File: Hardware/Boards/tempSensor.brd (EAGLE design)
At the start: 17.4 x 17.8 mm, 6 parts, among them IC1 DS1820

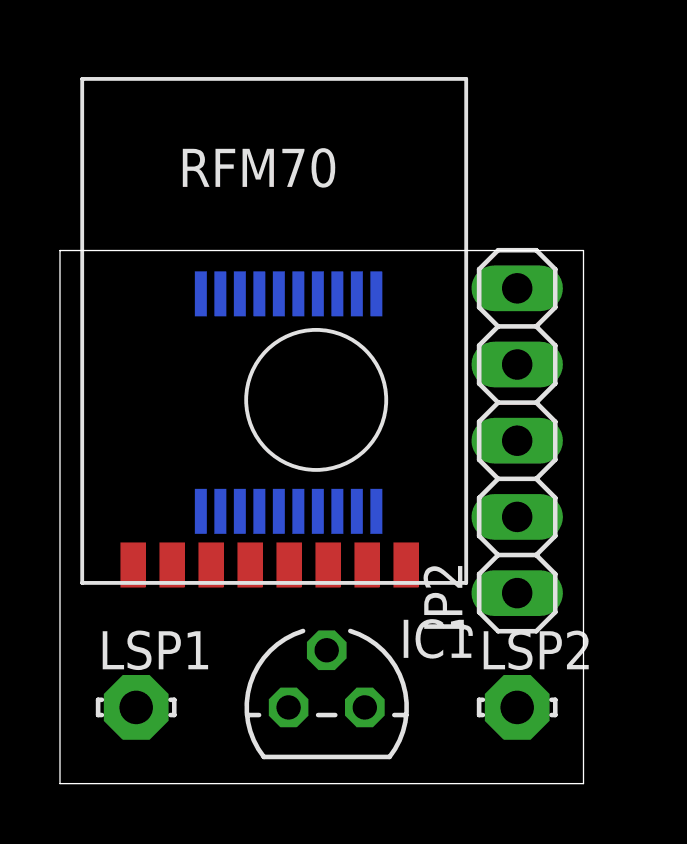
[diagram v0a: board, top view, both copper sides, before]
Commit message: a
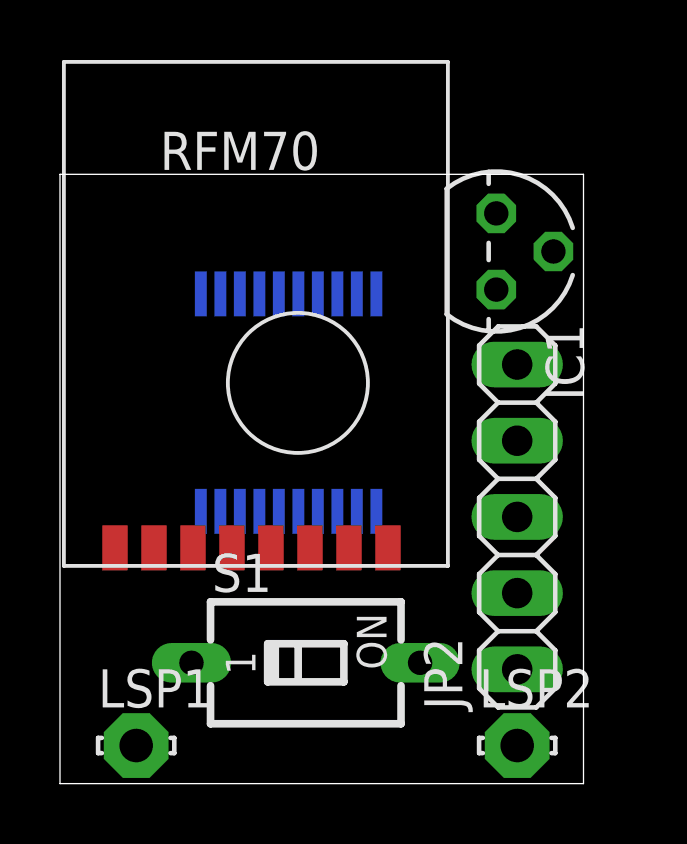
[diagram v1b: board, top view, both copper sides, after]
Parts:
- added S1: (no value), switch-dil:SD4-01
- moved IC1 16.2 mm to (14.5, 17.7), turned to 270 degrees
- moved JP2 2.54 mm to (15.2, 8.89)
- moved LSP1 1.27 mm to (2.54, 1.27)
- moved LSP2 1.27 mm to (15.2, 1.27)
- moved U$1 0.83 mm to (1.93, 22.2)
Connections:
- new net N$2: S1.2, U$2.3
- net N$5: now also S1.1
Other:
- board size 17.4 x 17.8 mm -> 17.4 x 20.3 mm
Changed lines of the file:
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@@
 <setting verticaltext="up"/>
 </settings>
-<grid distance="0.05" unitdist="inch" unit="inch" style="lines" multiple="1" display="no" altdistance="0.025" altunitdist="inch" altunit="inch"/>
+<grid distance="0.003125" unitdist="mic" unit="mm" style="lines" multiple="1" display="no" altdistance="0.025" altunitdist="inch" altunit="inch"/>
 <layers>
 <layer number="1" name="Top" color="4" fill="1" visible="yes" active="yes"/>
@@
 <plain>
 <wire x1="0" y1="0" x2="17.45" y2="0" width="0" layer="20"/>
-<wire x1="17.45" y1="0" x2="17.45" y2="17.77" width="0" layer="20"/>
-<wire x1="17.45" y1="17.77" x2="0" y2="17.77" width="0" layer="20"/>
-<wire x1="0" y1="17.77" x2="0" y2="0" width="0" layer="20"/>
+<wire x1="17.45" y1="0" x2="17.45" y2="20.31" width="0" layer="20"/>
+<wire x1="17.45" y1="20.31" x2="0" y2="20.31" width="0" layer="20"/>
+<wire x1="0" y1="20.31" x2="0" y2="0" width="0" layer="20"/>
 </plain>
 <attributes>
@@
 </autorouter>
 <elements>
-<element name="U$1" library="rfm70" package="RFM70" value="RFM70" x="2.54" y="21.59"/>
+<element name="U$1" library="rfm70" package="RFM70" value="RFM70" x="1.929840625" y="22.157171875"/>
 <element name="U$2" library="microchip" package="SSOP20" value="PIC16F690" x="7.62" y="12.7" rot="MR0"/>
-<element name="JP2" library="pinhead" package="1X05" value="Prog" x="15.24" y="11.43" rot="R90"/>
-<element name="IC1" library="ds1820" package="TO-92" value="DS1820" x="8.89" y="2.54"/>
-<element name="LSP1" library="solpad" package="LSP11" value="LSP11" x="2.54" y="2.54"/>
-<element name="LSP2" library="solpad" package="LSP11" value="LSP11" x="15.24" y="2.54"/>
+<element name="JP2" library="pinhead" package="1X05" value="Prog" x="15.24" y="8.89" rot="R90"/>
+<element name="IC1" library="ds1820" package="TO-92" value="DS1820" x="14.542675" y="17.7377375" rot="R270"/>
+<element name="LSP1" library="solpad" package="LSP11" value="LSP11" x="2.54" y="1.27"/>
+<element name="LSP2" library="solpad" package="LSP11" value="LSP11" x="15.24" y="1.27"/>
+<element name="S1" library="switch-dil" package="SD4-01" value="" x="8.192675" y="4.027234375" rot="R270">
+<attribute name="OC_NEWARK" value="unknown" x="8.192675" y="4.027234375" size="1.778" layer="27" rot="R270" display="off"/>
+<attribute name="MPN" value="" x="8.192675" y="4.027234375" size="1.778" layer="27" rot="R270" display="off"/>
+<attribute name="MF" value="" x="8.192675" y="4.027234375" size="1.778" layer="27" rot="R270" display="off"/>
+<attribute name="OC_FARNELL" value="unknown" x="8.192675" y="4.027234375" size="1.778" layer="27" rot="R270" display="off"/>
+</element>
 </elements>
 <signals>
@@
 <contactref element="IC1" pad="1"/>
 <contactref element="LSP2" pad="MP"/>
-<wire x1="10.545" y1="16.325" x2="2.44" y2="7.29" width="0" layer="19" extent="1-1"/>
-<wire x1="15.24" y1="11.43" x2="10.545" y2="16.325" width="0" layer="19" extent="1-1"/>
-<wire x1="7.62" y1="2.54" x2="15.24" y2="11.43" width="0" layer="19" extent="1-1"/>
-<wire x1="15.24" y1="2.54" x2="7.62" y2="2.54" width="0" layer="19" extent="1-1"/>
+<contactref element="S1" pad="1"/>
+<wire x1="15.24" y1="8.89" x2="10.545" y2="16.325" width="0" layer="19" extent="16-16"/>
+<wire x1="15.24" y1="1.27" x2="15.24" y2="8.89" width="0" layer="19" extent="1-1"/>
+<wire x1="14.542675" y1="19.0077375" x2="15.24" y2="1.27" width="0" layer="19" extent="1-1"/>
+<wire x1="1.829840625" y1="7.857171875" x2="14.542675" y2="19.0077375" width="0" layer="19" extent="1-1"/>
+<wire x1="4.382675" y1="4.027234375" x2="1.829840625" y2="7.857171875" width="0" layer="19" extent="1-1"/>
 </signal>
 <signal name="N$12">
 <contactref element="U$1" pad="MISO"/>
 <contactref element="U$2" pad="13"/>
-<wire x1="5.995" y1="16.325" x2="10.24" y2="7.29" width="0" layer="19" extent="1-1"/>
+<wire x1="5.995" y1="16.325" x2="9.629840625" y2="7.857171875" width="0" layer="19" extent="1-1"/>
 </signal>
 <signal name="N$17">
@@
 <contactref element="JP2" pad="2"/>
 <contactref element="LSP1" pad="MP"/>
-<wire x1="10.545" y1="9.075" x2="3.74" y2="7.29" width="0" layer="19" extent="1-1"/>
-<wire x1="15.24" y1="8.89" x2="10.545" y2="9.075" width="0" layer="19" extent="1-1"/>
-<wire x1="2.54" y1="2.54" x2="15.24" y2="8.89" width="0" layer="19" extent="1-1"/>
+<wire x1="10.545" y1="9.075" x2="3.129840625" y2="7.857171875" width="0" layer="19" extent="1-1"/>
+<wire x1="15.24" y1="6.35" x2="10.545" y2="9.075" width="0" layer="19" extent="1-1"/>
+<wire x1="2.54" y1="1.27" x2="15.24" y2="6.35" width="0" layer="19" extent="1-1"/>
 </signal>
 <signal name="N$18">
 <contactref element="U$2" pad="19"/>
 <contactref element="JP2" pad="4"/>
-<wire x1="9.895" y1="16.325" x2="15.24" y2="13.97" width="0" layer="19" extent="1-1"/>
+<wire x1="9.895" y1="16.325" x2="15.24" y2="11.43" width="0" layer="19" extent="1-1"/>
 </signal>
 <signal name="N$19">
 <contactref element="U$2" pad="18"/>
 <contactref element="JP2" pad="5"/>
-<wire x1="9.245" y1="16.325" x2="15.24" y2="16.51" width="0" layer="19" extent="1-1"/>
+<wire x1="9.245" y1="16.325" x2="15.24" y2="13.97" width="0" layer="19" extent="1-1"/>
 </signal>
 <signal name="N$16">
 <contactref element="U$2" pad="17"/>
 <contactref element="U$1" pad="CE"/>
-<wire x1="8.595" y1="16.325" x2="5.04" y2="7.29" width="0" layer="19" extent="1-1"/>
+<wire x1="8.595" y1="16.325" x2="4.429840625" y2="7.857171875" width="0" layer="19" extent="1-1"/>
 </signal>
 <signal name="N$20">
 <contactref element="U$2" pad="16"/>
 <contactref element="U$1" pad="CSN"/>
-<wire x1="7.945" y1="16.325" x2="6.34" y2="7.29" width="0" layer="19" extent="1-1"/>
+<wire x1="7.945" y1="16.325" x2="5.729840625" y2="7.857171875" width="0" layer="19" extent="1-1"/>
 </signal>
 <signal name="N$21">
 <contactref element="U$2" pad="14"/>
 <contactref element="U$1" pad="IRQ"/>
-<wire x1="6.645" y1="16.325" x2="11.54" y2="7.29" width="0" layer="19" extent="1-1"/>
+<wire x1="6.645" y1="16.325" x2="10.929840625" y2="7.857171875" width="0" layer="19" extent="1-1"/>
 </signal>
 <signal name="N$22">
 <contactref element="U$2" pad="11"/>
 <contactref element="U$1" pad="SCK"/>
-<wire x1="4.695" y1="16.325" x2="7.64" y2="7.29" width="0" layer="19" extent="1-1"/>
+<wire x1="4.695" y1="16.325" x2="7.029840625" y2="7.857171875" width="0" layer="19" extent="1-1"/>
 </signal>
 <signal name="N$23">
 <contactref element="U$2" pad="9"/>
 <contactref element="U$1" pad="MOSI"/>
-<wire x1="5.345" y1="9.075" x2="8.94" y2="7.29" width="0" layer="19" extent="1-1"/>
+<wire x1="5.345" y1="9.075" x2="8.329840625" y2="7.857171875" width="0" layer="19" extent="1-1"/>
 </signal>
 <signal name="N$25">
 <contactref element="U$2" pad="4"/>
 <contactref element="JP2" pad="1"/>
-<wire x1="8.595" y1="9.075" x2="15.24" y2="6.35" width="0" layer="19" extent="1-1"/>
+<wire x1="8.595" y1="9.075" x2="15.24" y2="3.81" width="0" layer="19" extent="1-1"/>
 </signal>
 <signal name="N$28">
@@
 <contactref element="IC1" pad="3"/>
 <contactref element="U$2" pad="5"/>
-<wire x1="7.945" y1="9.075" x2="10.16" y2="2.54" width="0" layer="19" extent="1-1"/>
+<wire x1="7.945" y1="9.075" x2="14.542675" y2="16.4677375" width="0" layer="19" extent="1-1"/>
 </signal>
 <signal name="N$1">
 <contactref element="IC1" pad="2"/>
 <contactref element="U$2" pad="2"/>
-<wire x1="9.895" y1="9.075" x2="8.89" y2="4.445" width="0" layer="19" extent="1-1"/>
+<wire x1="9.895" y1="9.075" x2="16.447675" y2="17.7377375" width="0" layer="19" extent="1-1"/>
+</signal>
+<signal name="N$2">
+<contactref element="S1" pad="2"/>
+<contactref element="U$2" pad="3"/>
+<wire x1="12.002675" y1="4.027234375" x2="9.245" y2="9.075" width="0" layer="19" extent="16-16"/>
 </signal>
 </signals>
